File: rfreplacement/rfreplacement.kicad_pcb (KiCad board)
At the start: 2 copper layers, 43.9 x 55.9 mm, 27 parts

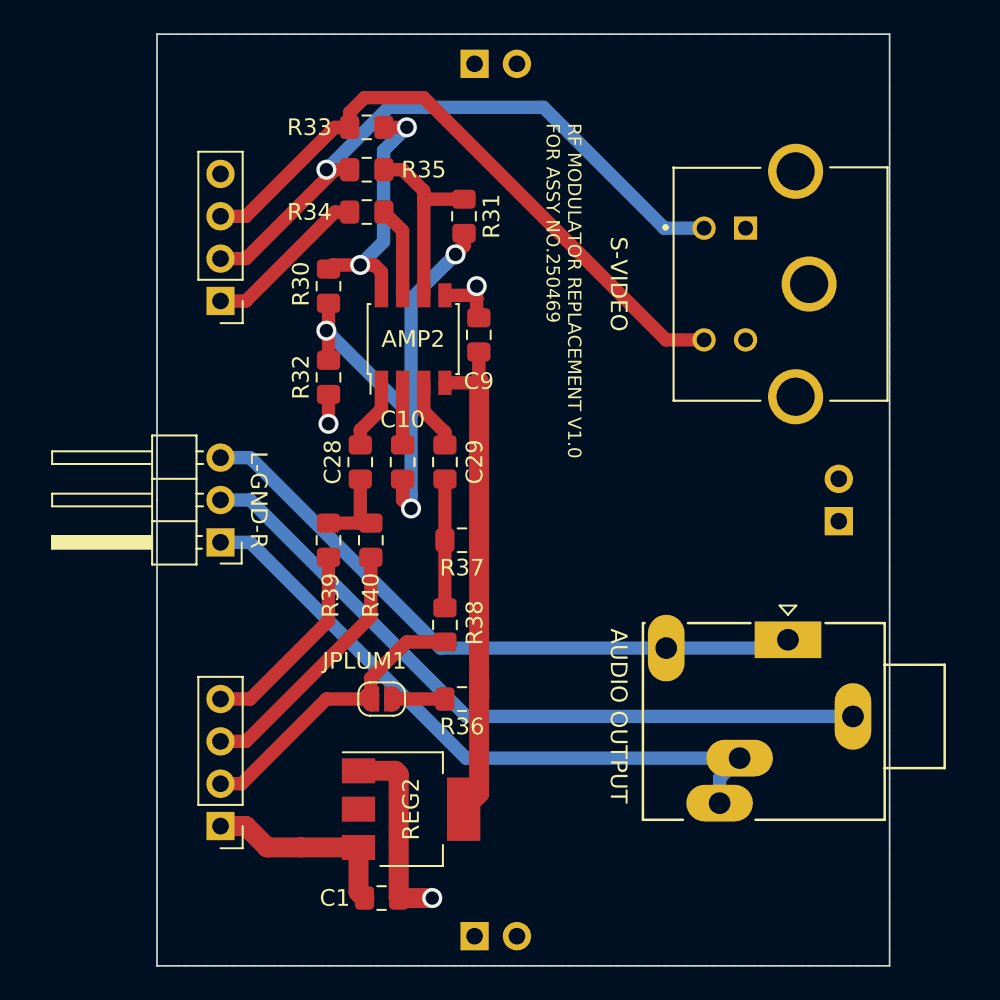
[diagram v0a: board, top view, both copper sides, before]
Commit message: PCB ver 1.2
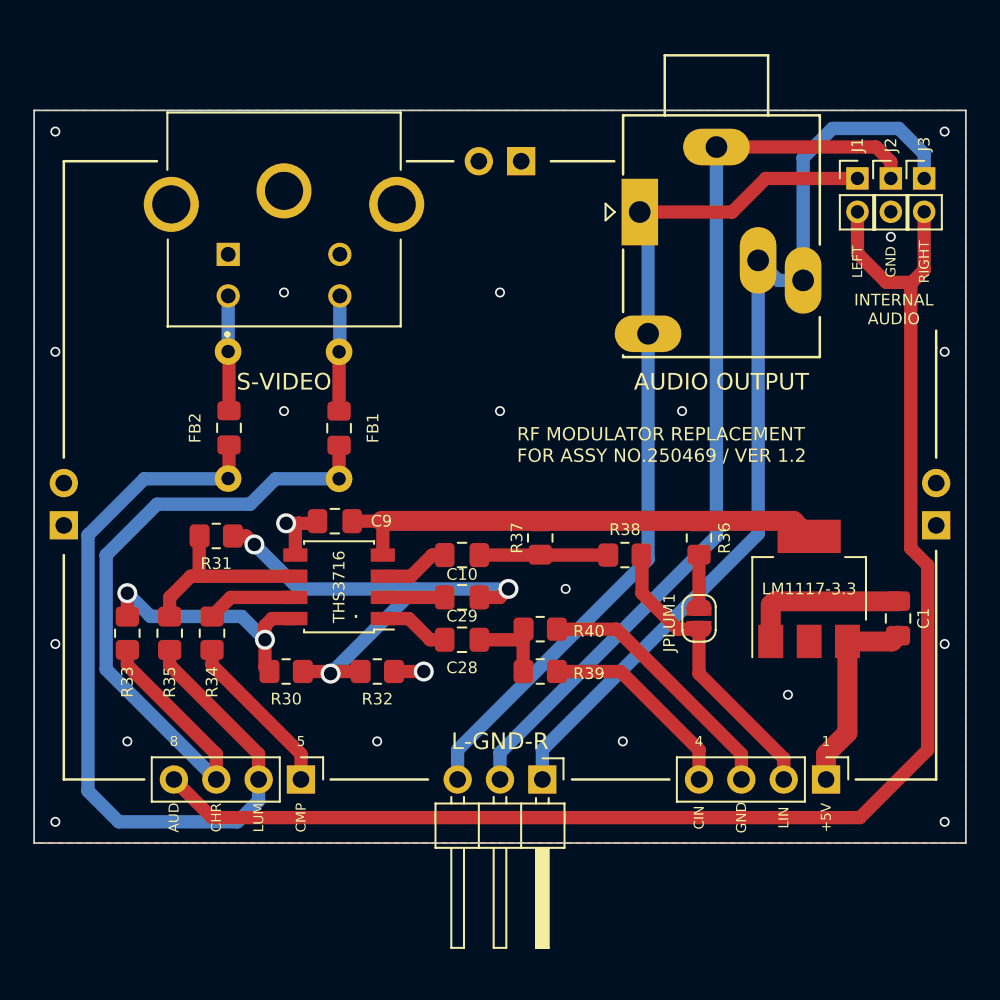
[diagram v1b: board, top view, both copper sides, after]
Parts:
- added FB1: Ferrite Bead, Inductor_SMD:L_0805_2012Metric_Pad1.15x1.40mm_HandSolder, F.Cu at (115.1, 78.7)
- added FB2: Ferrite Bead, Inductor_SMD:L_0805_2012Metric_Pad1.15x1.40mm_HandSolder, F.Cu at (108.5, 78.7)
- added FB3: Alternative THT, Resistor_THT:R_Axial_DIN0207_L6.3mm_D2.5mm_P7.62mm_Horizontal, B.Cu at (115.1, 74.2)
- added FB4: Alternative THT, Resistor_THT:R_Axial_DIN0207_L6.3mm_D2.5mm_P7.62mm_Horizontal, B.Cu at (108.4, 74.2)
- added J1: Conn_01x02, Connector_PinHeader_2.00mm:PinHeader_1x02_P2.00mm_Vertical, F.Cu at (146.2, 63.8)
- added J2: Conn_01x02, Connector_PinHeader_2.00mm:PinHeader_1x02_P2.00mm_Vertical, F.Cu at (148.2, 63.8)
- added J3: Conn_01x02, Connector_PinHeader_2.00mm:PinHeader_1x02_P2.00mm_Vertical, F.Cu at (150.2, 63.8)
- added REF**: OSHW-Logo2_9.8x8mm_SilkScreen, Symbol:OSHW-Logo2_9.8x8mm_SilkScreen, B.Cu at (106.2, 91.4)
- added REF**: KiCad-Logo2_5mm_SilkScreen, Symbol:KiCad-Logo2_5mm_SilkScreen, B.Cu at (141.2, 80.5)
- C1, C10, C28, C29, C9: footprint Capacitor_SMD:C_0805_2012Metric_Pad1.15x1.40mm_HandSolder -> Capacitor_SMD:C_0805_2012Metric_Pad1.18x1.45mm_HandSolder
- R30, R31, R32, R33, R34, R35, R36, R37, R38, R39, R40: footprint Resistor_SMD:R_0805_2012Metric_Pad1.15x1.40mm_HandSolder -> Resistor_SMD:R_0805_2012Metric_Pad1.20x1.40mm_HandSolder
- moved GND2 37.1 mm to (150.9, 84.6), turned to 0 degrees
- moved GND3 37.1 mm to (98.6, 84.6), turned to 0 degrees
- moved RFCONC2 36.4 mm to (144.3, 99.8), turned to -90 degrees
- moved C1 35.2 mm to (148.6, 90.2), turned to -90 degrees
- moved R33 33.6 mm to (102.4, 91.0), turned to 90 degrees
- moved R35 30.2 mm to (104.9, 91.0), turned to 90 degrees
- moved RFCONC1 29.1 mm to (112.8, 99.8), turned to -90 degrees
- moved GND1 28.8 mm to (126.0, 62.7), turned to 90 degrees
- moved S-VIDEO1 27.7 mm to (111.8, 68.3), turned to 0 degrees
- moved LM1117-3.3 27.3 mm to (143.3, 88.4), turned to 90 degrees
- moved STEREO_OUT1 27.2 mm to (133.1, 65.8), turned to -90 degrees
- moved R34 26.9 mm to (107.4, 91.0), turned to -90 degrees
- moved R31 24.3 mm to (107.7, 85.2), turned to 0 degrees
- moved AUDIO_OUT1 24.0 mm to (127.3, 99.8), turned to -90 degrees
- moved R30 23.3 mm to (111.9, 93.3), turned to 180 degrees
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- renumbered REG2 to LM1117-3.3, AMP2 to THS3716
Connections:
- net +12V renamed +5V
- LM1117-3.3 pad 2: (no net) -> unconnected-(REG2-Pad2)
- RFCONC1 pad 4: (no net) -> /AUDIO_OUT
- S-VIDEO1 pad 3: /LUMA_OUT -> Net-(FB2-Pad2)
- S-VIDEO1 pad 4: /CHROMA_OUT -> Net-(FB1-Pad2)
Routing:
- net /AUDIO_OUT: track 0.00 -> 87.4 mm
- net /AUDIO_RIGHT: track 39.7 -> 57.1 mm
- net /LUMA_OUT: track 37.2 -> 50.0 mm, vias 1 -> 0
- net /AUDIO_LEFT: track 41.2 -> 52.2 mm
- net /AUDIO_GND: track 44.5 -> 55.1 mm
- net Net-(FB1-Pad2): track 0.00 -> 6.86 mm
- net Net-(FB2-Pad2): track 0.00 -> 6.84 mm
- net /CHROMA_OUT: track 38.5 -> 44.0 mm
- net GNDA: track 33.3 -> 31.2 mm, vias 3 -> 21
- net /3V3X: track 31.2 -> 29.9 mm
- added copper zone on F.Cu, net GNDA
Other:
- board size 43.9 x 55.9 mm -> 55.9 x 43.9 mm
- net class Default removed
- net class power removed
- board text added: "+5V"
- board text added: "."
- board text added: "1"
- board text added: "4"
- board text added: "5"
- board text added: "8"
- board text added: "AUD"
- board text added: "C64 Video Enhancement, Analog Only github.com/c0pperdragon PCB design for ASSY NO.250469 / Ver 1.2 by Pawel Mandes / devzine.pl github.com/pmandes/C64-RF-Modulator"
- board text added: "CHR"
- board text added: "CHROMINANCE"
- board text added: "CIN"
- board text added: "CMP"
- board text added: "GND"
- board text added: "INTERNAL AUDIO"
- board text added: "LEFT"
- board text added: "LIN"
- board text added: "LUM"
- board text added: "LUMINANCE"
- board text added: "RF MODULATOR REPLACEMENT FOR ASSY NO.250469 / VER 1.2"
- board text added: "RIGHT"
- board text removed: "C64 Video Enhancement, Analog Only github.com/c0pperdragon PCB design for ASSY NO.250469 by Pawel Mandes / devzine.pl github.com/pmandes/C64-RF-Modulator"
- board text removed: "RF MODULATOR REPLACEMENT V1.0 FOR ASSY NO.250469"
